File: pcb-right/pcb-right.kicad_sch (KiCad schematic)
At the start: 92 parts, among them J1 Conn_01x04_Pin, J2 Conn_01x02_Pin, J3 Conn_01x06_MountingPin, SW1 SW_Push, SW2 Rotary_Encoder_Default, U1 XC6206PxxxMR, U2 STM32F401RCTx, Y1 8MHz

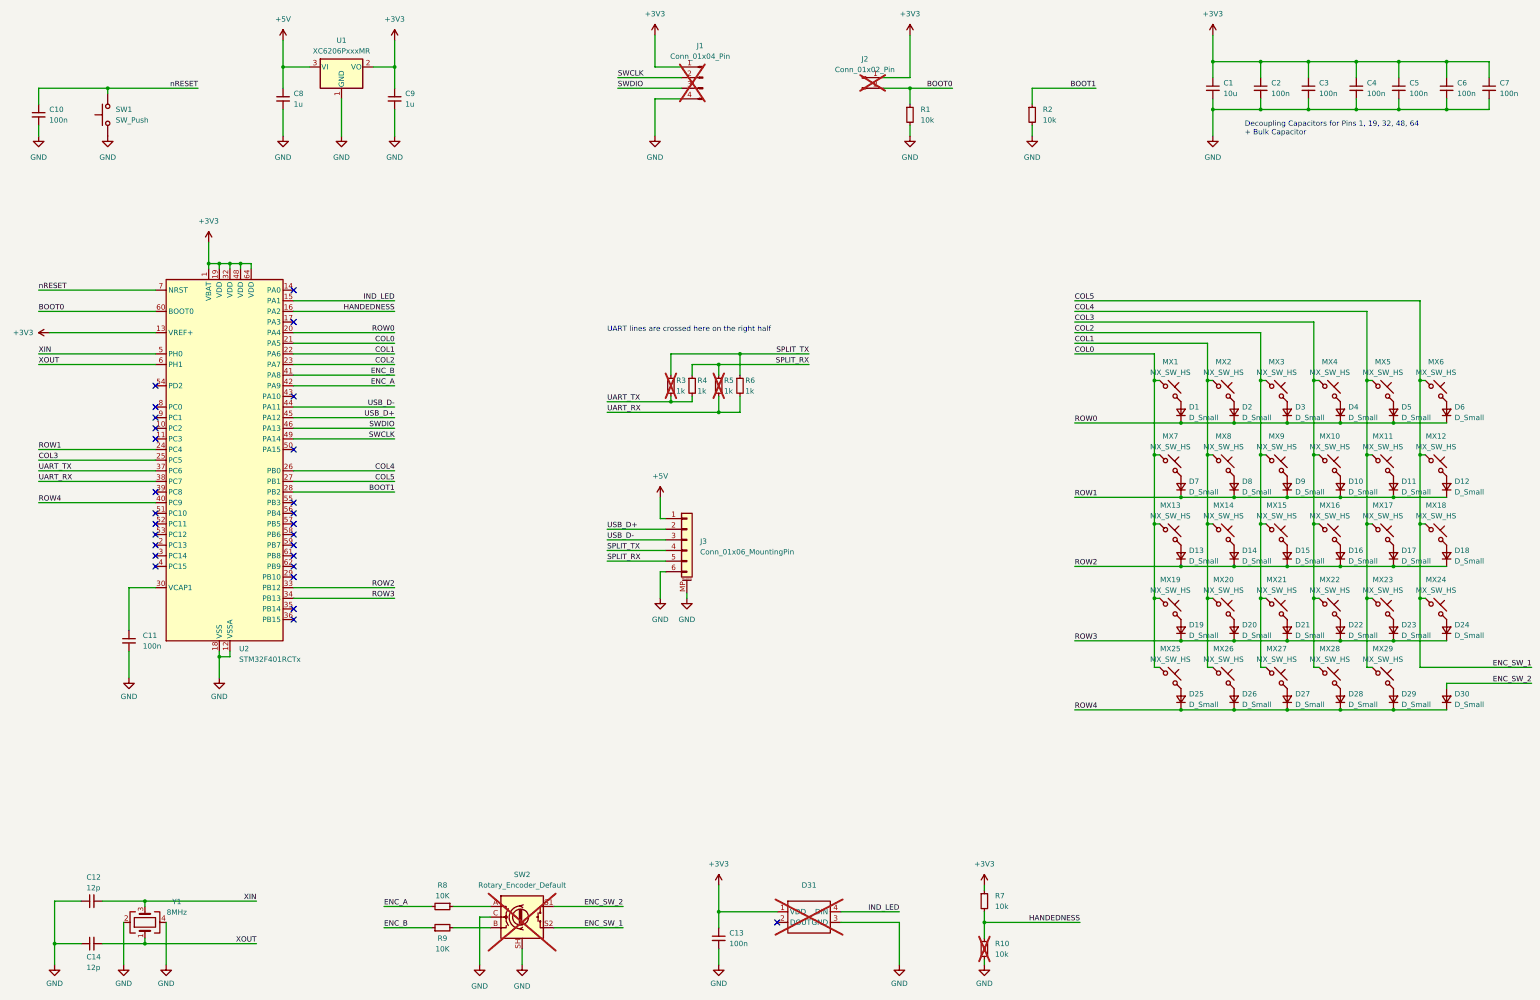
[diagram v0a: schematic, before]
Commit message: intermediate save
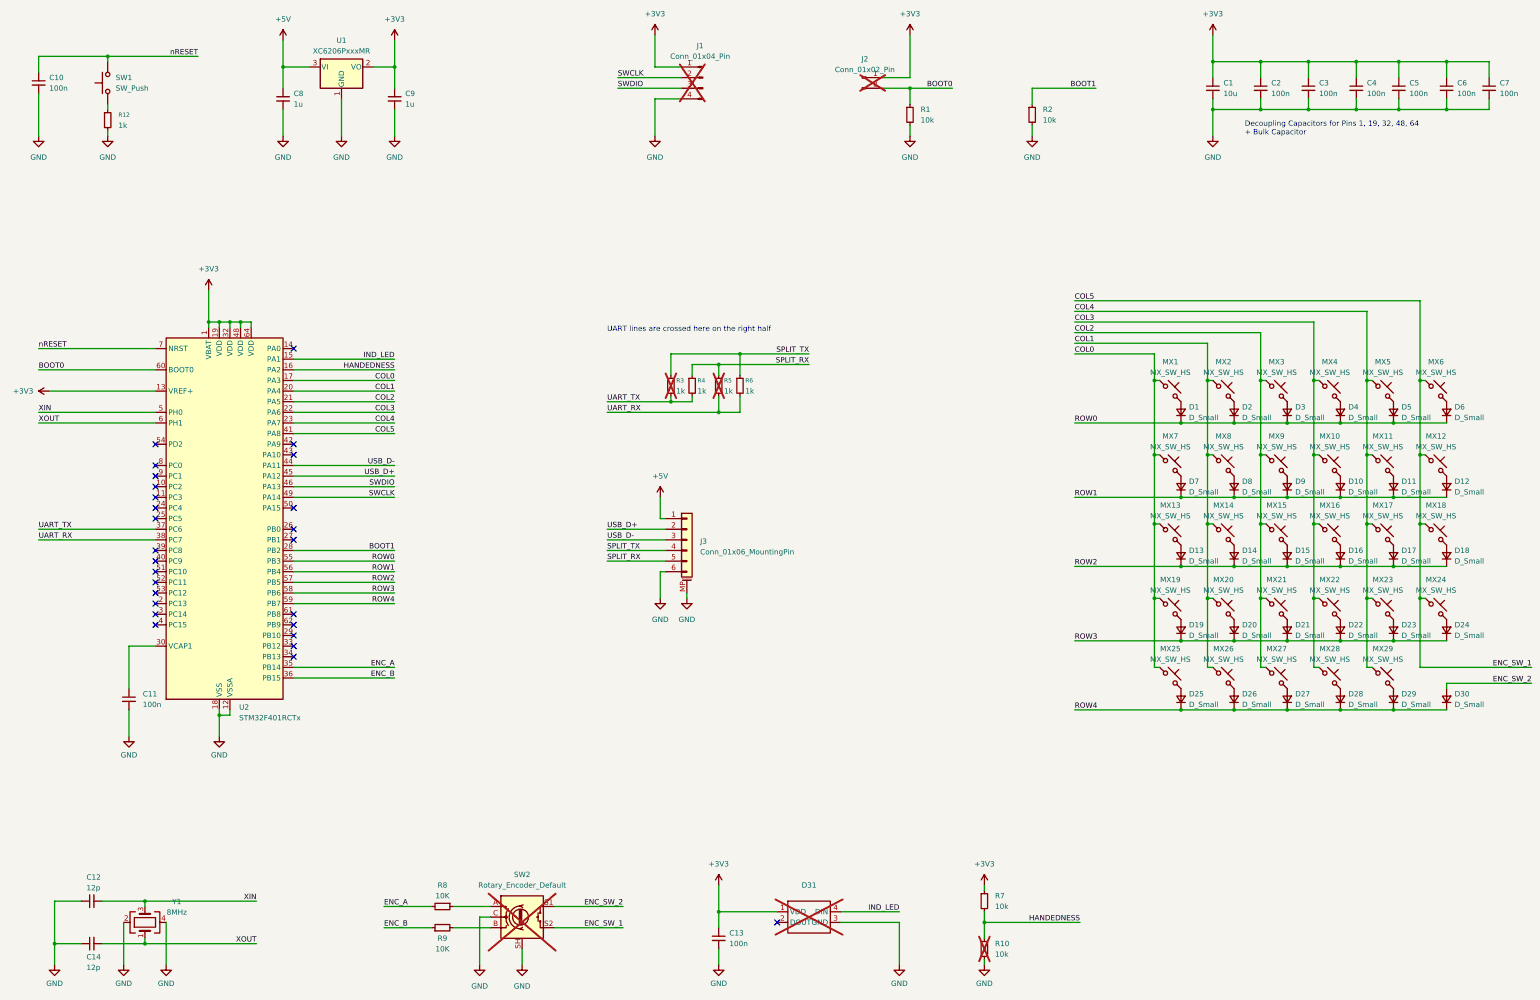
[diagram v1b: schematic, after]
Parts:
- added R12: 1k, symbol Device:R_Small
- R3, R5: footprint Resistor_SMD:R_0402_1005Metric -> (none); now in the parts list
- R4, R6: footprint Resistor_SMD:R_0603_1608Metric_Pad0.98x0.95mm_HandSolder -> (none)
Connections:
- net COL0: now also U2.17 (PA3); no longer U2.21 (PA5)
- net COL1: now also U2.20 (PA4); no longer U2.22 (PA6)
- net COL2: now also U2.21 (PA5); no longer U2.23 (PA7)
- net COL3: now also U2.22 (PA6); no longer U2.25 (PC5)
- net COL4: now also U2.23 (PA7); no longer U2.26 (PB0)
- net COL5: now also U2.41 (PA8); no longer U2.27 (PB1)
- net ENC_A: now also U2.35 (PB14); no longer U2.42 (PA9)
- net ENC_B: now also U2.36 (PB15); no longer U2.41 (PA8)
- net GND: now also R12.2; no longer SW1.1
- net ROW0: now also U2.55 (PB3); no longer U2.20 (PA4)
- net ROW1: now also U2.56 (PB4); no longer U2.24 (PC4)
- net ROW2: now also U2.57 (PB5); no longer U2.33 (PB12)
- net ROW3: now also U2.58 (PB6); no longer U2.34 (PB13)
- net ROW4: now also U2.59 (PB7); no longer U2.40 (PC9)
- new net: R12.1, SW1.1
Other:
- moved on the sheet: C10, C11, SW1, U2
